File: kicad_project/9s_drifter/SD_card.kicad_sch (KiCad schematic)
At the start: 1 part, among them J1 SD_Card_Device

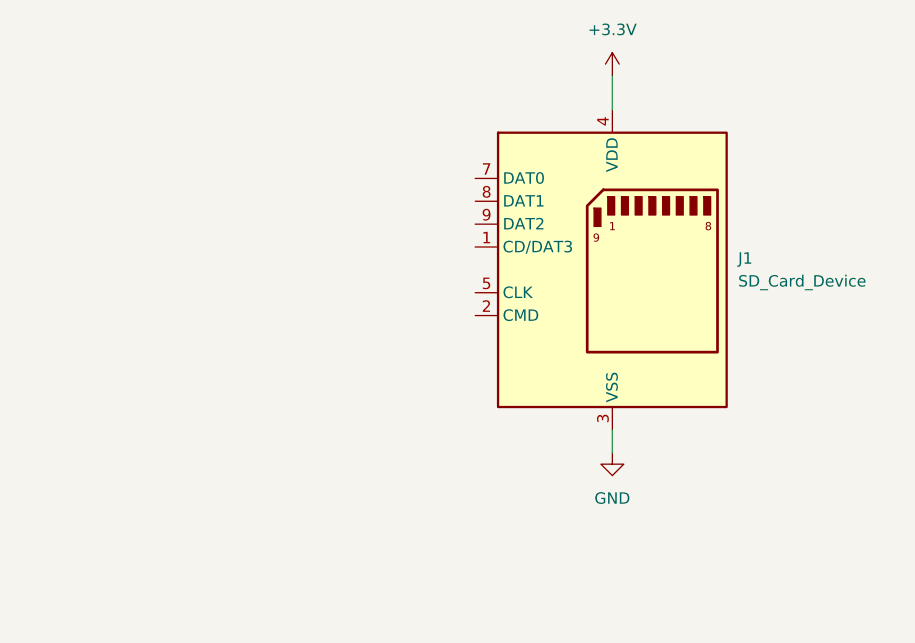
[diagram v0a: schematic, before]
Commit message: Update
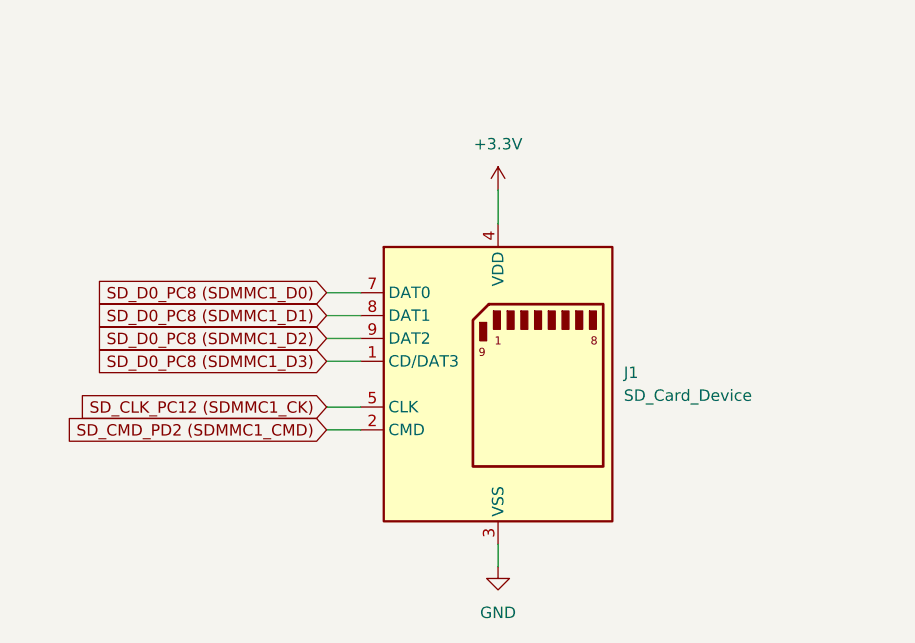
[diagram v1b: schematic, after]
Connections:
- net SD_D0_PC8 (SDMMC1_D3): now reaches J1.1 (CD/DAT3)
- net SD_CMD_PD2 (SDMMC1_CMD): now reaches J1.2 (CMD)
- net SD_CLK_PC12 (SDMMC1_CK): now reaches J1.5 (CLK)
- net SD_D0_PC8 (SDMMC1_D0): now reaches J1.7 (DAT0)
- net SD_D0_PC8 (SDMMC1_D1): now reaches J1.8 (DAT1)
- net SD_D0_PC8 (SDMMC1_D2): now reaches J1.9 (DAT2)
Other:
- moved on the sheet: J1
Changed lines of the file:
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@@
 	(wire
 		(pts
-			(xy 88.9 58.42) (xy 88.9 60.96)
-		)
-		(stroke
-			(width 0)
-			(type default)
-		)
-	)
-	(wire
-		(pts
-			(xy 88.9 19.05) (xy 88.9 22.86)
-		)
-		(stroke
-			(width 0)
-			(type default)
+			(xy 76.2 71.12) (xy 76.2 73.66)
+		)
+		(stroke
+			(width 0)
+			(type default)
+		)
+	)
+	(wire
+		(pts
+			(xy 57.15 43.18) (xy 60.96 43.18)
+		)
+		(stroke
+			(width 0)
+			(type default)
+		)
+	)
+	(wire
+		(pts
+			(xy 57.15 48.26) (xy 60.96 48.26)
+		)
+		(stroke
+			(width 0)
+			(type default)
+		)
+	)
+	(wire
+		(pts
+			(xy 57.15 45.72) (xy 60.96 45.72)
+		)
+		(stroke
+			(width 0)
+			(type default)
+		)
+	)
+	(wire
+		(pts
+			(xy 57.15 58.42) (xy 60.96 58.42)
+		)
+		(stroke
+			(width 0)
+			(type default)
+		)
+	)
+	(wire
+		(pts
+			(xy 57.15 50.8) (xy 60.96 50.8)
+		)
+		(stroke
+			(width 0)
+			(type default)
+		)
+	)
+	(wire
+		(pts
+			(xy 57.15 55.88) (xy 60.96 55.88)
+		)
+		(stroke
+			(width 0)
+			(type default)
+		)
+	)
+	(wire
+		(pts
+			(xy 76.2 31.75) (xy 76.2 35.56)
+		)
+		(stroke
+			(width 0)
+			(type default)
+		)
+	)
+	(global_label "SD_D0_PC8 (SDMMC1_D1)"
+		(shape input)
+		(at 57.15 45.72 180)
+		(fields_autoplaced yes)
+		(effects
+			(font
+				(size 1.27 1.27)
+			)
+			(justify right)
+		)
+		(property "Intersheetrefs" "${INTERSHEET_REFS}"
+			(at 29.5512 45.72 0)
+			(effects
+				(font
+					(size 1.27 1.27)
+				)
+				(justify right)
+				(hide yes)
+			)
+		)
+	)
+	(global_label "SD_D0_PC8 (SDMMC1_D3)"
+		(shape input)
+		(at 57.15 50.8 180)
+		(fields_autoplaced yes)
+		(effects
+			(font
+				(size 1.27 1.27)
+			)
+			(justify right)
+		)
+		(property "Intersheetrefs" "${INTERSHEET_REFS}"
+			(at 29.5512 50.8 0)
+			(effects
+				(font
+					(size 1.27 1.27)
+				)
+				(justify right)
+				(hide yes)
+			)
+		)
+	)
+	(global_label "SD_CLK_PC12 (SDMMC1_CK)"
+		(shape input)
+		(at 57.15 55.88 180)
+		(fields_autoplaced yes)
+		(effects
+			(font
+				(size 1.27 1.27)
+			)
+			(justify right)
+		)
+		(property "Intersheetrefs" "${INTERSHEET_REFS}"
+			(at 27.1926 55.88 0)
+			(effects
+				(font
+					(size 1.27 1.27)
+				)
+				(justify right)
+				(hide yes)
+			)
+		)
+	)
+	(global_label "SD_D0_PC8 (SDMMC1_D0)"
+		(shape input)
+		(at 57.15 43.18 180)
+		(fields_autoplaced yes)
+		(effects
+			(font
+				(size 1.27 1.27)
+			)
+			(justify right)
+		)
+		(property "Intersheetrefs" "${INTERSHEET_REFS}"
+			(at 29.5512 43.18 0)
+			(effects
+				(font
+					(size 1.27 1.27)
+				)
+				(justify right)
+				(hide yes)
+			)
+		)
+	)
+	(global_label "SD_D0_PC8 (SDMMC1_D2)"
+		(shape input)
+		(at 57.15 48.26 180)
+		(fields_autoplaced yes)
+		(effects
+			(font
+				(size 1.27 1.27)
+			)
+			(justify right)
+		)
+		(property "Intersheetrefs" "${INTERSHEET_REFS}"
+			(at 29.5512 48.26 0)
+			(effects
+				(font
+					(size 1.27 1.27)
+				)
+				(justify right)
+				(hide yes)
+			)
+		)
+	)
+	(global_label "SD_CMD_PD2 (SDMMC1_CMD)"
+		(shape input)
+		(at 57.15 58.42 180)
+		(fields_autoplaced yes)
+		(effects
+			(font
+				(size 1.27 1.27)
+			)
+			(justify right)
+		)
+		(property "Intersheetrefs" "${INTERSHEET_REFS}"
+			(at 26.5274 58.42 0)
+			(effects
+				(font
+					(size 1.27 1.27)
+				)
+				(justify right)
+				(hide yes)
+			)
 		)
 	)
 	(symbol
 		(lib_id "power:GND")
-		(at 88.9 60.96 0)
+		(at 76.2 73.66 0)
 		(unit 1)
 		(exclude_from_sim no)
@@
 		(fields_autoplaced yes)
 		(property "Reference" "#PWR012"
-			(at 88.9 67.31 0)
+			(at 76.2 80.01 0)
 			(effects
 				(font
@@
 		)
 		(property "Value" "GND"
-			(at 88.9 66.04 0)
+			(at 76.2 78.74 0)
 			(effects
 				(font
@@
 		)
 		(property "Footprint" ""
-			(at 88.9 60.96 0)
+			(at 76.2 73.66 0)
 			(effects
 				(font
@@
 		)
 		(property "Datasheet" ""
-			(at 88.9 60.96 0)
+			(at 76.2 73.66 0)
 			(effects
 				(font
@@
 		)
 		(property "Description" "Power symbol creates a global label with name \"GND\" , ground"
-			(at 88.9 60.96 0)
+			(at 76.2 73.66 0)
 			(effects
 				(font
@@
 	(symbol
 		(lib_id "power:+3.3V")
-		(at 88.9 19.05 0)
+		(at 76.2 31.75 0)
 		(unit 1)
 		(exclude_from_sim no)
@@
 		(fields_autoplaced yes)
 		(property "Reference" "#PWR013"
-			(at 88.9 22.86 0)
+			(at 76.2 35.56 0)
 			(effects
 				(font
@@
 		)
 		(property "Value" "+3.3V"
-			(at 88.9 13.97 0)
+			(at 76.2 26.67 0)
 			(effects
 				(font
@@
 		)
 		(property "Footprint" ""
-			(at 88.9 19.05 0)
+			(at 76.2 31.75 0)
 			(effects
 				(font
@@
 		)
 		(property "Datasheet" ""
-			(at 88.9 19.05 0)
+			(at 76.2 31.75 0)
 			(effects
 				(font
@@
 		)
 		(property "Description" "Power symbol creates a global label with name \"+3.3V\""
-			(at 88.9 19.05 0)
+			(at 76.2 31.75 0)
 			(effects
 				(font
@@
 	(symbol
 		(lib_id "Connector:SD_Card_Device")
-		(at 88.9 40.64 0)
+		(at 76.2 53.34 0)
 		(unit 1)
 		(exclude_from_sim no)
@@
 		(fields_autoplaced yes)
 		(property "Reference" "J1"
-			(at 102.87 39.3699 0)
+			(at 90.17 52.0699 0)
 			(effects
 				(font
@@
 		)
 		(property "Value" "SD_Card_Device"
-			(at 102.87 41.9099 0)
+			(at 90.17 54.6099 0)
 			(effects
 				(font
@@
 		)
 		(property "Footprint" ""
-			(at 88.9 40.64 0)
+			(at 76.2 53.34 0)
 			(effects
 				(font
@@
 		)
 		(property "Datasheet" "http://www.convict.lu/pdf/ProdManualSDCardv1.9.pdf"
-			(at 88.9 40.64 0)
+			(at 76.2 53.34 0)
 			(effects
 				(font
@@
 		)
 		(property "Description" "SD card device/card"
-			(at 88.9 40.64 0)
-			(effects
-				(font
+			(at 76.2 53.34 0)
+			(effects
+				(font
